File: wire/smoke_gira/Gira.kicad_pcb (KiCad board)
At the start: 2 copper layers, 38 x 65 mm, 33 parts, among them IC1 MEGA8-PTQFP, Q1 2N7002, Q2 2N7002, Q3 2N7002

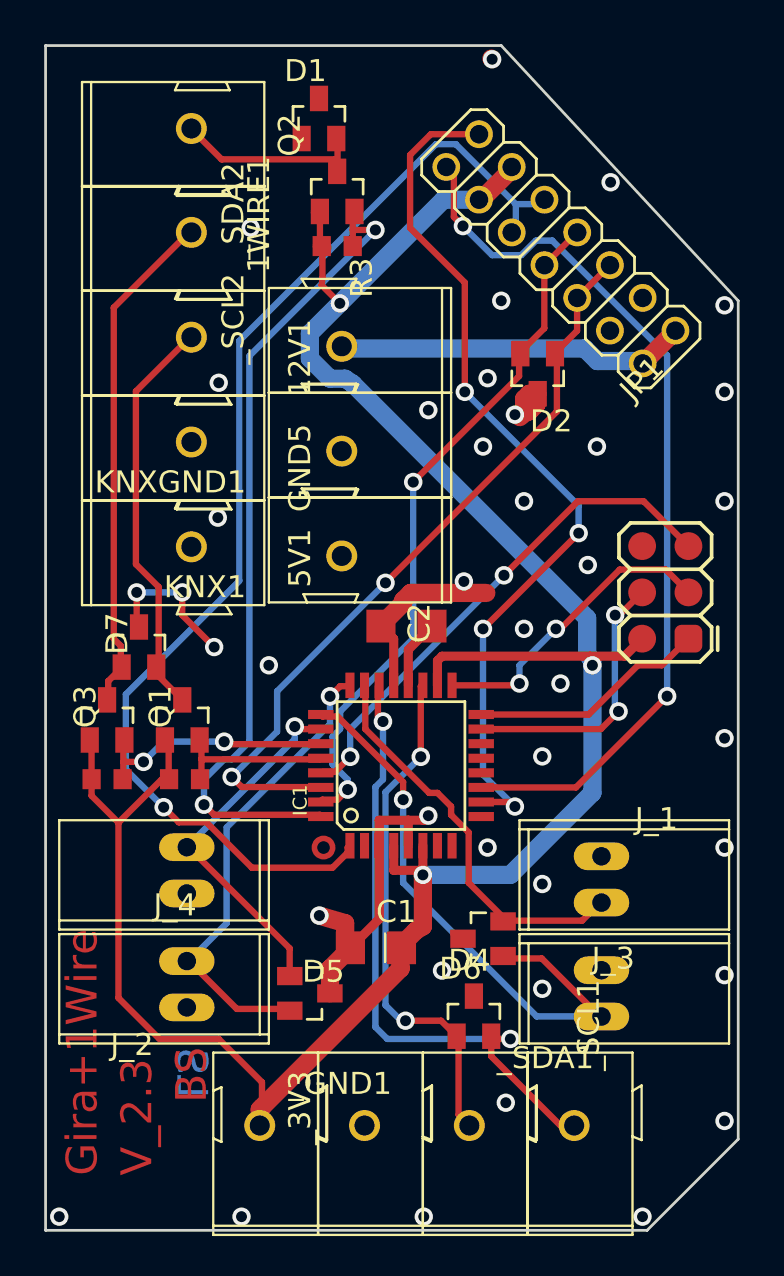
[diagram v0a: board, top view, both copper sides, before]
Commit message: Re-worked the Gira thing
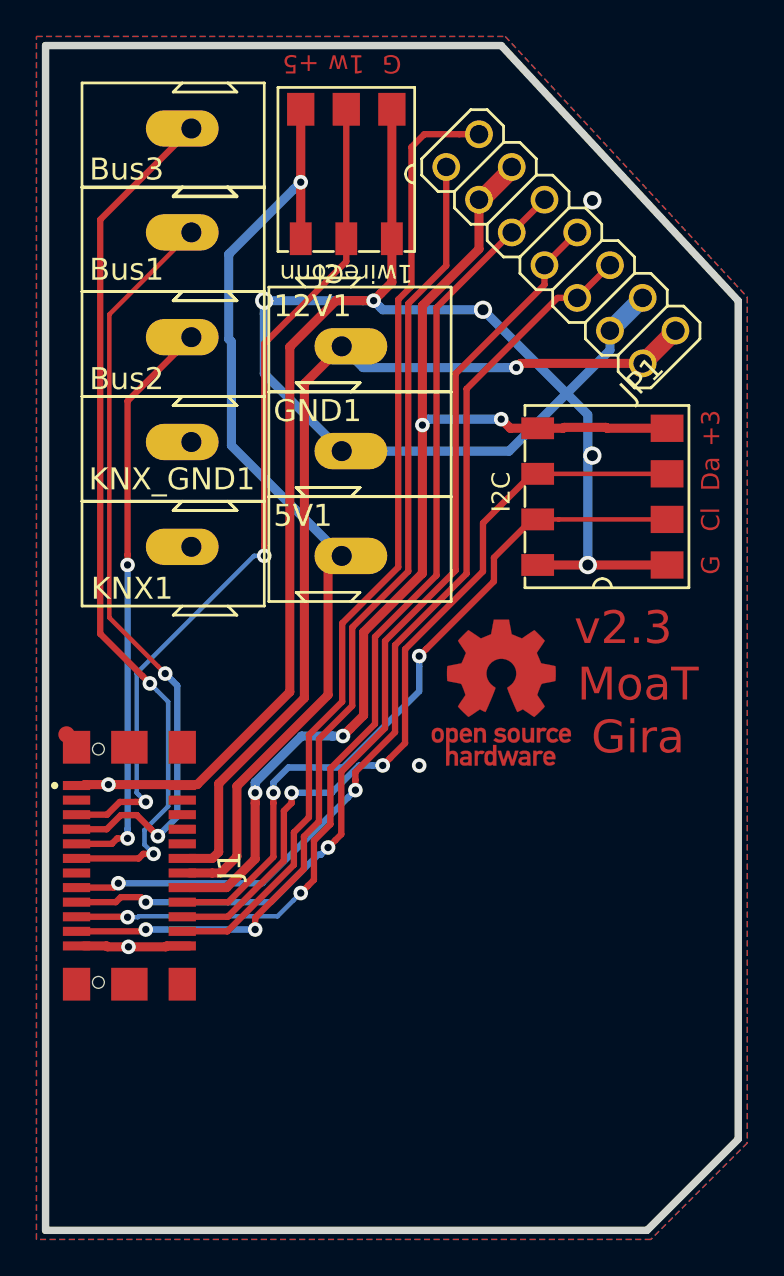
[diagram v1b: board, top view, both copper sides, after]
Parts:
- removed 1WIRE1, GND5, KNXGND1, _3V3, _GND1, _SCL1, _SCL2, _SDA1, _SDA2: WAGO_243, Gira:WAGO_243
- removed C1, C2: CP1206, Gira:CP1206
- removed D1, D2, D4, D5, D6, D7: ESD_DIODES, Gira:SOT23
- removed IC1: MEGA8-PTQFP, Gira:TQFP32-08
- removed J_1, J_2, J_3, J_4: PINHD-1X2LEVER, Gira:1X02_GN
- removed Q1, Q2, Q3: 2N7002, Gira:SOT23
- removed R1, R2, R3: R-EU_R0603, Gira:R0603
- removed U$1: AVR_SPI_PRG_6PAD, Gira:2X3_PAD
- added Bus1: WAGO_243, localstuff:Wago_Terminal_243, F.Cu at (137.5, 82.8)
- added Bus2: WAGO_243, localstuff:Wago_Terminal_243, F.Cu at (137.5, 88.5)
- added Bus3: WAGO_243, localstuff:Wago_Terminal_243, F.Cu at (137.5, 77.1)
- added GND1: WAGO_243, localstuff:Wago_Terminal_243, F.Cu at (145.8, 94.8)
- added J1: Moat_Bus_wire, localstuff:TE_1775014_socket, F.Cu at (134.1, 117.5)
- added J2: 1wireConn, localstuff:AVX_9276_3Pin, F.Cu at (146.0, 79.5)
- added J3: I2C, localstuff:AVX_9276_4Pin, F.Cu at (160.1, 97.2)
- added KNX_GND1: WAGO_243, localstuff:Wago_Terminal_243, F.Cu at (137.5, 94.3)
- added REF**: OSHW-Logo_7.5x8mm_Copper, Symbol:OSHW-Logo_7.5x8mm_Copper, F.Cu at (154.5, 108.0)
- 12V1, 5V1, KNX1: footprint Gira:WAGO_243 -> localstuff:Wago_Terminal_243
- JP1: value PINHD-2X7 -> Gira
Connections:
- net Net-(D2-Pad1) renamed /TxD
- net Net-(D2-Pad2) renamed /RxD
- net Net-(IC1-Pad1) renamed /Unk_1
- JP1 pad 1: Net-(12V1-PadP$1) -> +12V
- JP1 pad 13: Net-(JP1-Pad13) -> /Unk_2
- JP1 pad 2: Net-(12V1-PadP$1) -> +12V
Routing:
- net +3V3: track 195.4 -> 63.3 mm, vias 7 -> 4
- net GND: track 40.7 -> 121.1 mm, vias 39 -> 9
- net /B2: track 74.7 -> 0.00 mm, vias 5 -> 0
- net +5V: track 0.00 -> 53.7 mm, vias 0 -> 1
- net /Unk_2: track 0.00 -> 53.3 mm
- net +12V: track 0.00 -> 51.9 mm, vias 0 -> 1
- net Net-(Bus3-Pad1): track 0.00 -> 48.1 mm, vias 0 -> 2
- net /1wire: track 0.00 -> 47.0 mm, vias 0 -> 2
- net Net-(IC1-Pad32): track 45.6 -> 0.00 mm, vias 2 -> 0
- net /SDA: track 0.00 -> 42.8 mm, vias 0 -> 2
- net Net-(Bus1-Pad1): track 0.00 -> 41.8 mm, vias 0 -> 2
- net /SCL: track 0.00 -> 39.2 mm, vias 0 -> 2
- net /B3: track 32.3 -> 0.00 mm, vias 1 -> 0
- net Net-(Bus2-Pad1): track 0.00 -> 31.5 mm, vias 0 -> 2
- net Net-(IC1-Pad29): track 28.2 -> 0.00 mm, vias 2 -> 0
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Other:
- net class Power added: clearance 0.3, trace_width 0.5, via_dia 0.8, via_drill 0.4
- board text added: "+3"
- board text added: "+5"
- board text added: "1w"
- board text added: "Cl"
- board text added: "Da"
- board text added: "G"
- board text added: "MoaT Gira"
- board text added: "v2.3"
- board text removed: "BS"
- board text removed: "Gira+1Wire"
- board text removed: "LS"
- board text removed: "V_2.3"
